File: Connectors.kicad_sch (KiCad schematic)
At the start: 22 parts, among them J1 KH-1.27PH180-1X4P-L7.2, J2 KH-1.27PH180-1X4P-L7.2, J3 2171750001, J401 B3U-3000P-B, U2 ICM-42688-P, U6 TJA1051T/3

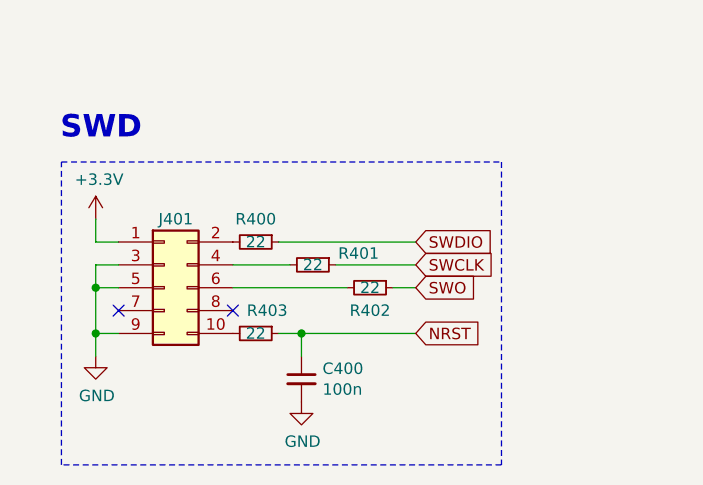
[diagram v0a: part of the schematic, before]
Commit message: Cleanup and check on JCLPCB
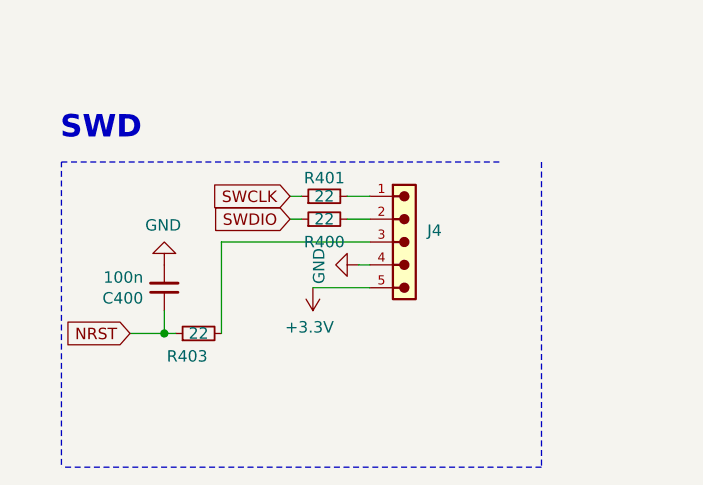
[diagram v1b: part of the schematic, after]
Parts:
- removed J401: B3U-3000P-B, Connector_PinHeader_1.27mm:PinHeader_2x05_P1.27mm_Vertical, symbol Connector_Generic:Conn_02x05_Odd_Even
- removed R402: 22, Resistor_SMD:R_0402_1005Metric, symbol Device:R_Small
- added J4: ZX-PZ2.54-1-5PZZ, CONN-HEADER-VERT-5POS-2.54MM:CONN-HEADER-VERT-5POS-2.54MM, symbol CONN-HEADER-VERT-5POS-2.54MM:6130XX11121_61300511121
- R19, R20: footprint Resistor_SMD:R_0402_1005Metric -> Resistor_SMD:R_0603_1608Metric
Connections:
- net +3.3V: now also J4.5
- net GND: now also J4.4
- net at R403.2: now also J4.3
- net at R400.2: now also J4.2
- net at R401.2: now also J4.1
- no-connect marks 8 -> 6
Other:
- moved on the sheet: C400, R400, R401, R403

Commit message: Version for JLCPCB
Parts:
- C10: footprint Capacitor_SMD:C_0201_0603Metric -> Capacitor_SMD:C_0402_1005Metric
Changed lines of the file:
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@@
 			)
 		)
-		(property "Footprint" "Capacitor_SMD:C_0201_0603Metric"
+		(property "Footprint" "Capacitor_SMD:C_0402_1005Metric"
 			(at 229.87 107.95 0)
 			(effects
